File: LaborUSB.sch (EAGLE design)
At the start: 13 parts

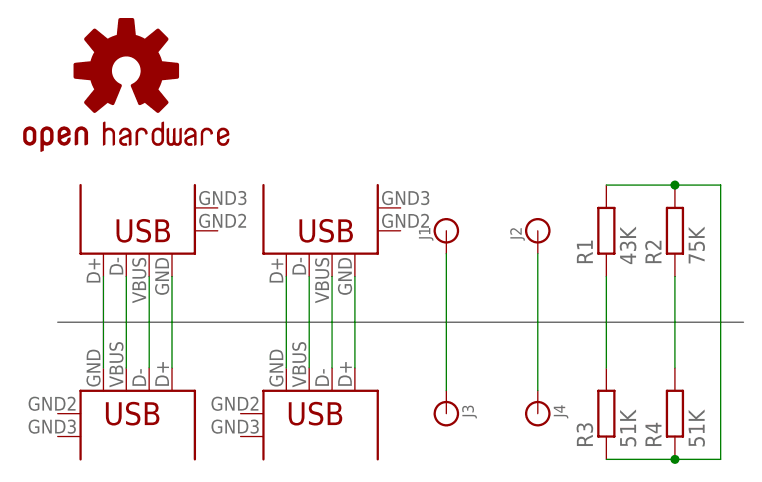
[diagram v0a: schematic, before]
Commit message: First prototype order
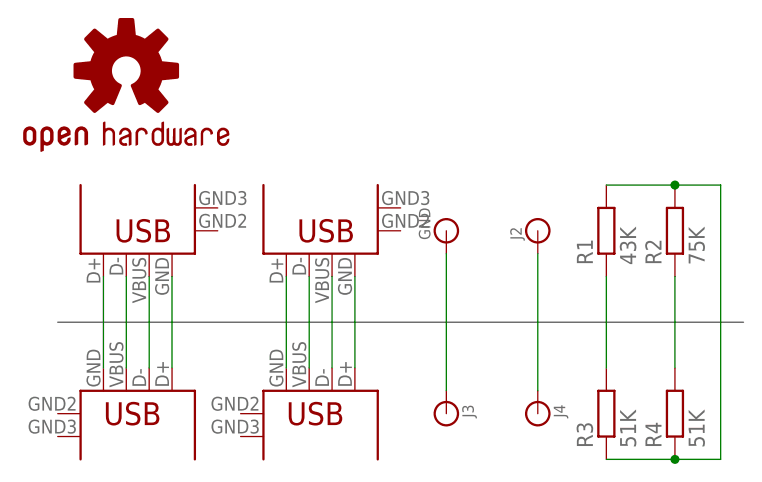
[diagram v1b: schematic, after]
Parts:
- renumbered J1 to GND
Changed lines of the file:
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@@
 </classes>
 <parts>
-<part name="J1" library="LaborUSB" deviceset="BANANA" device=""/>
+<part name="GND" library="LaborUSB" deviceset="BANANA" device=""/>
 <part name="J2" library="LaborUSB" deviceset="BANANA" device=""/>
 <part name="J3" library="LaborUSB" deviceset="BANANA" device=""/>
@@
 </plain>
 <instances>
-<instance part="J1" gate="G$1" x="40.64" y="165.1" rot="R90"/>
+<instance part="GND" gate="G$1" x="40.64" y="165.1" rot="R90"/>
 <instance part="J2" gate="G$1" x="50.8" y="165.1" rot="R90"/>
 <instance part="J3" gate="G$1" x="40.64" y="144.78" rot="R270"/>
@@
 <segment>
 <wire x1="40.64" y1="162.56" x2="40.64" y2="154.94" width="0.1524" layer="91"/>
-<pinref part="J1" gate="G$1" pin="1"/>
+<pinref part="GND" gate="G$1" pin="1"/>
 </segment>
 <segment>
